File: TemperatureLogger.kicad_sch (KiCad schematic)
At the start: 16 parts, among them J1 I2C, J3 Micro_SD_Card, SW1 RESET, SW2 A, SW3 B, SW4 MODE, SW5 POWER, U1 bme280, U2 UA78M33_TO252, U3 esp-01m, U4 TTL, U5 tp4056

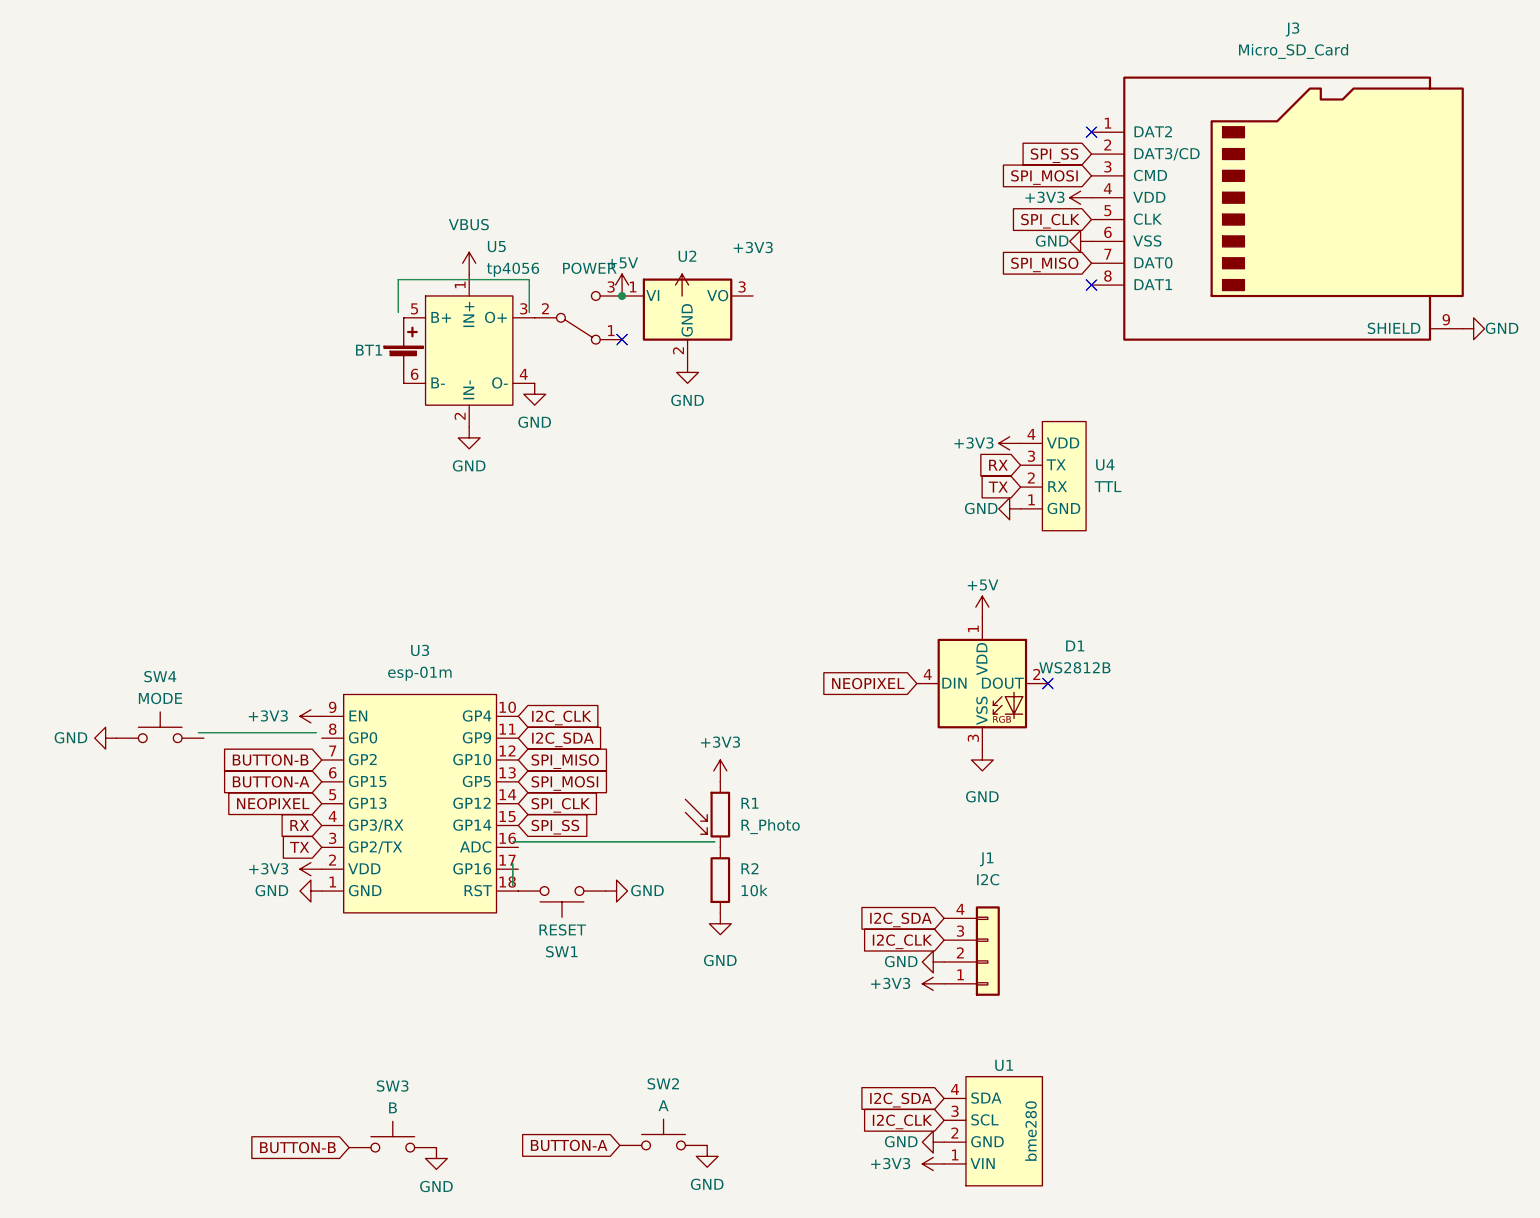
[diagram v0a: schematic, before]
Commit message: First routing
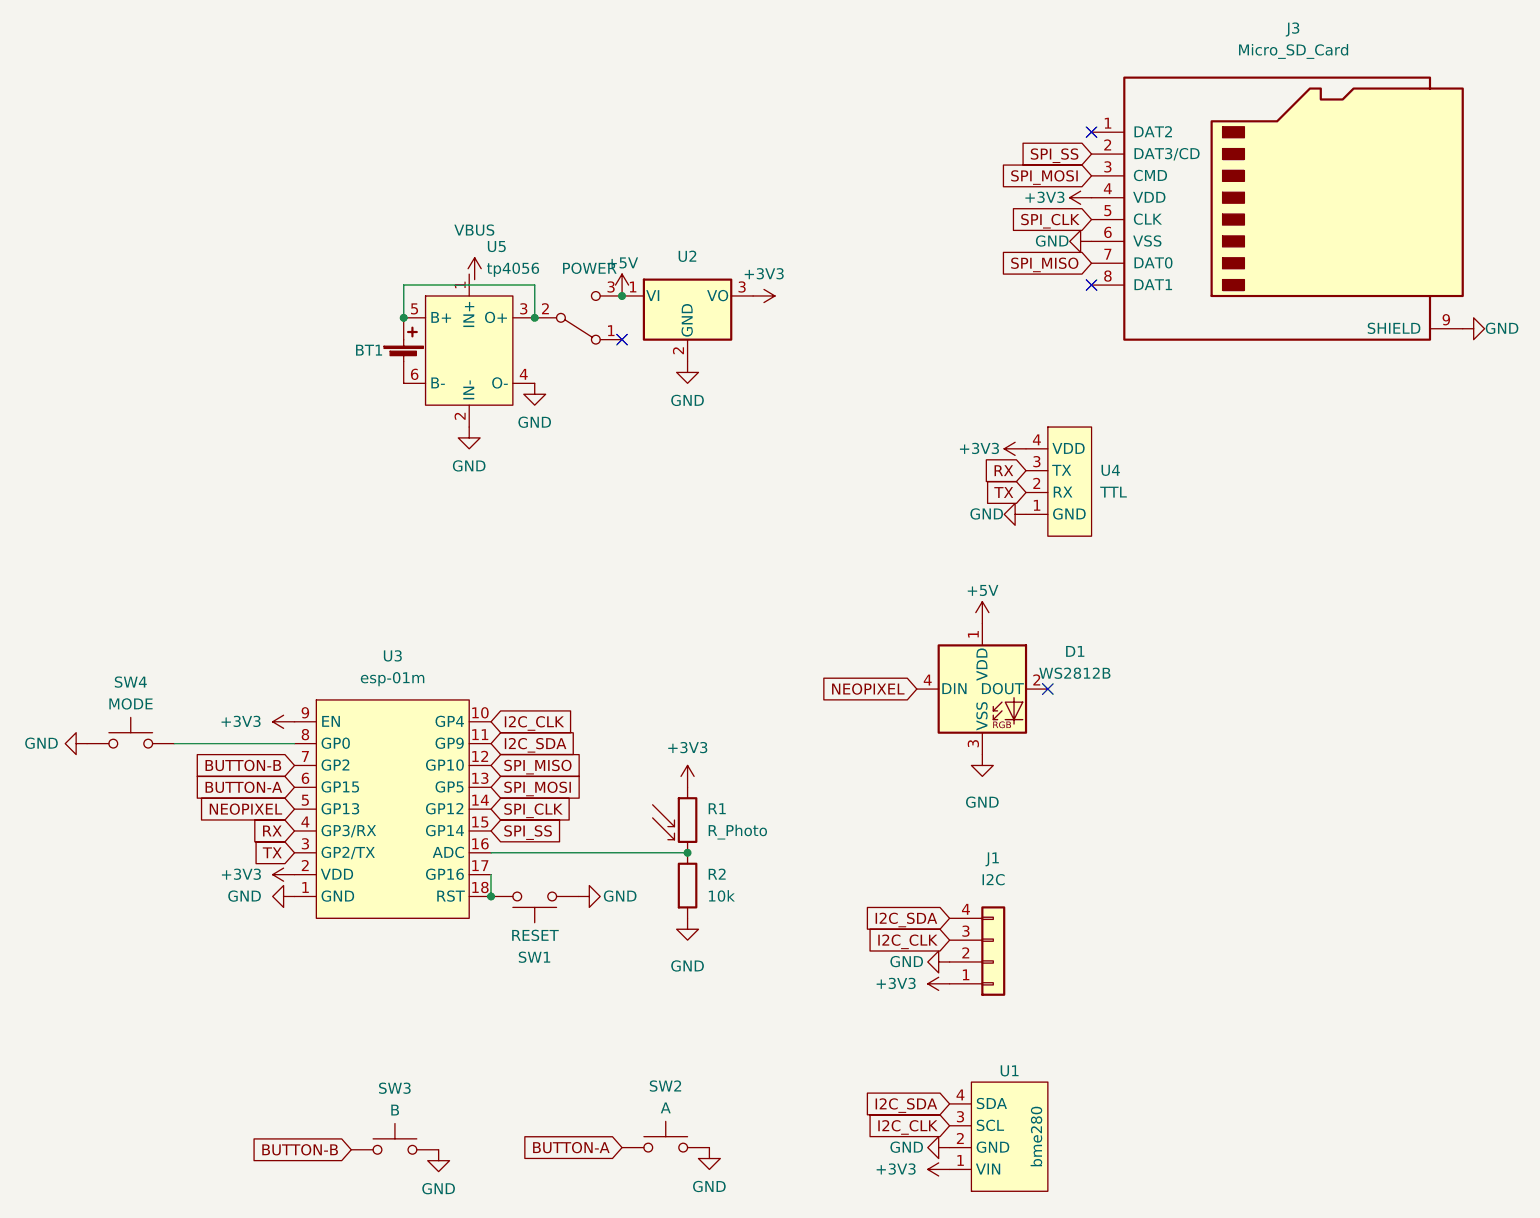
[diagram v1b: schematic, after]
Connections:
- net +3V3: now also U2.3 (VO)
- net VBUS: no longer U5.1 (IN+)
- net at SW4.2: now also U3.8 (GP0)
- net at R1.2, R2.1: now also U3.16 (ADC)
- net at SW5.2 (B), U5.3 (O+): now also BT1.1 (+), U5.5 (B+)
- net at U3.17 (GP16): now also SW1.2, U3.18 (RST)
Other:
- moved on the sheet: D1, J1, R1, R2, SW1, SW4, U1, U3, U4
